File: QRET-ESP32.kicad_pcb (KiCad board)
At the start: 4 copper layers, 109 x 77.2 mm, 130 parts, among them J1 Conn_01x04, J10 Conn_01x04, J2 Conn_01x02, J3 Conn_02x01, J4 Conn_01x02, J5 Conn_01x02, J6 Conn_01x02, J7 Conn_02x04_Counter_Clockwise, J8 Conn_02x04_Counter_Clockwise, J9 Conn_01x04, Q3 BSS138, Q4 BSS138, Q5 BSS138, U1 ESP32-S2-DevKitC-1, U2 LM3880-1AA, U3 LMR33630BDDA, U4 LMR33630BDDA, U5 TPS78533QKVURQ1, U6 TPS78450QDBVRQ1, U7 ADS112C04, U8 ADS112C04, U9 ADS112C04

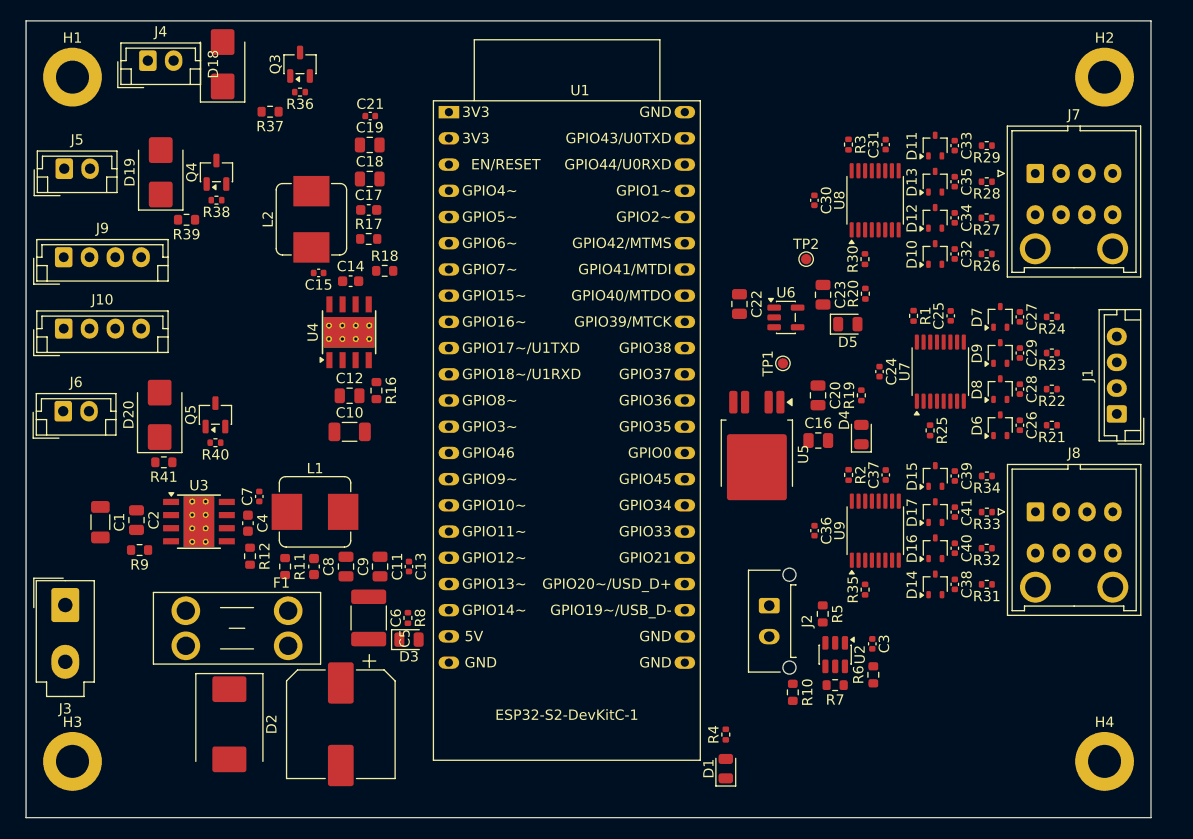
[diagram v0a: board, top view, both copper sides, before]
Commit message: Second draft of placement and wiring.
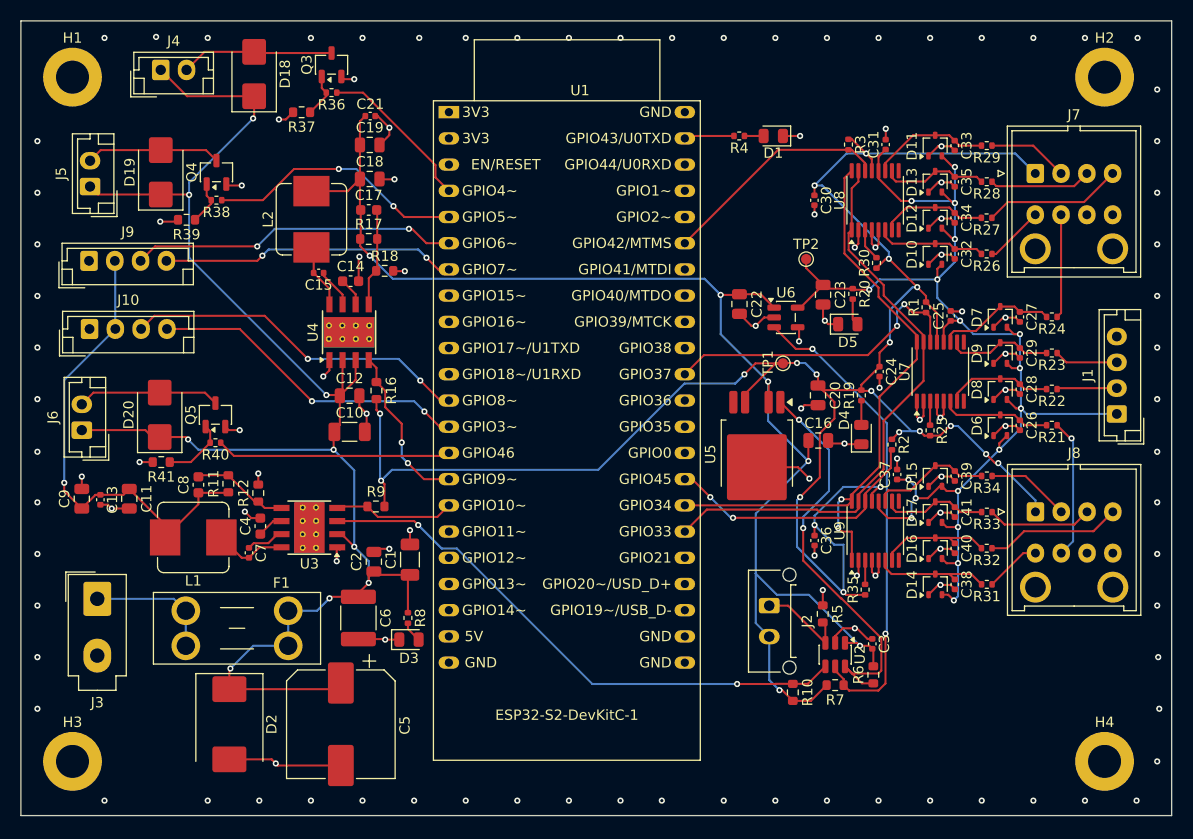
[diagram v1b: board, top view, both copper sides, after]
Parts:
- moved D1 61.5 mm to (159.8, 64.5), turned to 180 degrees
- moved R4 58.0 mm to (156.5, 64.5), turned to 180 degrees
- moved C13 30.6 mm to (94.6, 99.8)
- moved C1 30.2 mm to (124.6, 105.5), turned to 90 degrees
- moved C9 26.4 mm to (92.8, 99.7), turned to 90 degrees
- moved C11 25.2 mm to (97.4, 99.7)
- moved C2 23.4 mm to (121.1, 105.8), turned to 90 degrees
- moved R9 23.3 mm to (121.3, 100.4), turned to 0 degrees
- moved C8 13.7 mm to (104.1, 98.3), turned to 90 degrees
- moved L1 12.1 mm to (103.6, 103.4), turned to 180 degrees
- moved U3 10.7 mm to (114.8, 102.5), turned to 180 degrees
- moved R11 9.72 mm to (107.0, 98.2), turned to 90 degrees
- moved R12 6.17 mm to (109.9, 99.1), turned to 90 degrees
- moved C7 5.55 mm to (109.0, 104.9), turned to -90 degrees
- moved R2 5.13 mm to (171.3, 94.4)
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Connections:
- J10 pad 1: +12V -> GND
- J10 pad 2: Fan_2_Control -> +12V
- J10 pad 3: Fan_2_PWM -> Fan_2_Control
- J10 pad 4: GND -> Fan_2_PWM
- J7 pad 1: Heat_1_Power -> +3.3V
- J8 pad 1: Heat_2_Power -> +3.3V
- J9 pad 1: +12V -> GND
- J9 pad 2: Fan_1_Control -> +12V
- J9 pad 3: Fan_1_PWM -> Fan_1_Control
- J9 pad 4: GND -> Fan_1_PWM
- U1 pad 27: /ESP32-Breakout/WIFI_IND -> unconnected-(U1-GPIO21-Pad27)
- U1 pad 30: unconnected-(U1-GPIO45-Pad30) -> DRDY3
- U1 pad 34: unconnected-(U1-GPIO37-Pad34) -> DRDY1
- U1 pad 37: DRDY3 -> unconnected-(U1-GPIO40/MTDO-Pad37)
- U1 pad 38: DRDY2 -> unconnected-(U1-GPIO41/MTDI-Pad38)
- U1 pad 39: DRDY1 -> DRDY2
- U1 pad 43: unconnected-(U1-GPIO43/U0TXD-Pad43) -> /ESP32-Breakout/WIFI_IND
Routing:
- net +3.3V: track 0.00 -> 204.8 mm, vias 0 -> 20
- net +24V: track 0.00 -> 154.0 mm, vias 0 -> 9
- net GND: track 0.00 -> 139.3 mm, vias 0 -> 120
- net /Power_Regulation/+5.3V: track 0.00 -> 132.8 mm, vias 0 -> 6
- net +5V: track 0.00 -> 126.2 mm, vias 0 -> 18
- net I2C_Clock: track 0.00 -> 62.4 mm, vias 0 -> 2
- net I2C_Data: track 0.00 -> 56.7 mm
- net /Power_Regulation/+12_EN: track 0.00 -> 54.5 mm, vias 0 -> 2
- net +12V: track 0.00 -> 46.9 mm, vias 0 -> 1
- net /Power_Regulation/+5V_EN: track 0.00 -> 46.7 mm, vias 0 -> 2
- net /Power_Regulation/+3.3V_EN: track 0.00 -> 39.6 mm, vias 0 -> 2
- net Fan_2_Control: track 0.00 -> 33.7 mm, vias 0 -> 2
- net Fan_1_Control: track 0.00 -> 31.7 mm, vias 0 -> 2
- net Fan_2_PWM: track 0.00 -> 31.2 mm, vias 0 -> 2
- net DRDY1: track 0.00 -> 30.4 mm, vias 0 -> 2
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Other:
- board size 109 x 77.2 mm -> 111.5 x 77 mm
